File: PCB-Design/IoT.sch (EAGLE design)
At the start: 11 parts, among them M2 ARDUINO-NANO-3.0, M3 WIRELESS-NRF24L01

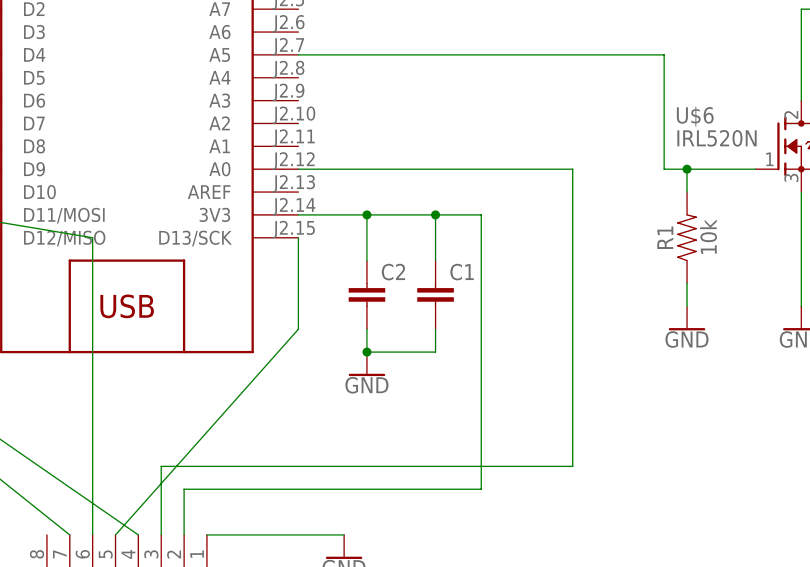
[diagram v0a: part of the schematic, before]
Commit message: Redone PCB on bottom only
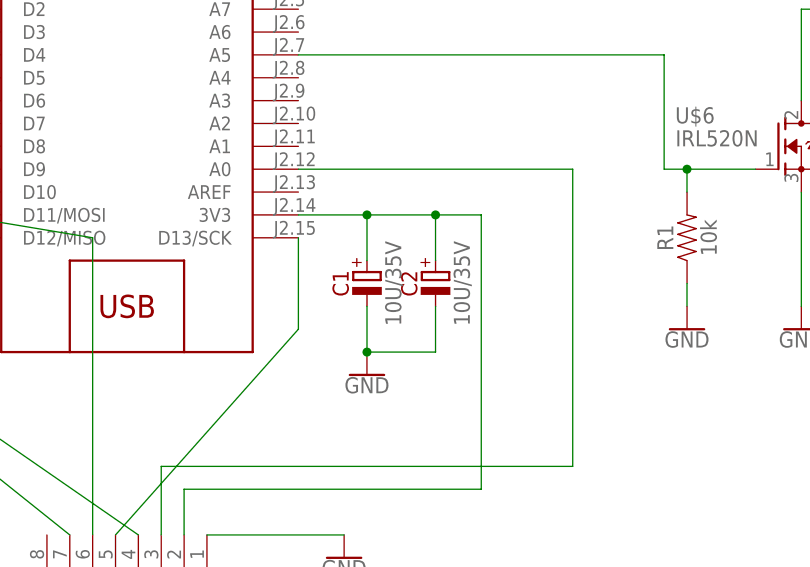
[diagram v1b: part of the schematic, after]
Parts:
- C1, C2: value (none) -> 10U/35V; device resistor:C-EU025-040X050 -> capacitors-electrolytic:10U/35V
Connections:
- removed net N$4: C1.1, C2.1, M2.3V3, M3.VCC
- new net N$2: C1.+, C2.+, M2.3V3, M3.VCC
- net GND: now also C1.-, C2.-; no longer C1.2, C2.2
